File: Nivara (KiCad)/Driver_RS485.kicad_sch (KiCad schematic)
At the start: 3 parts

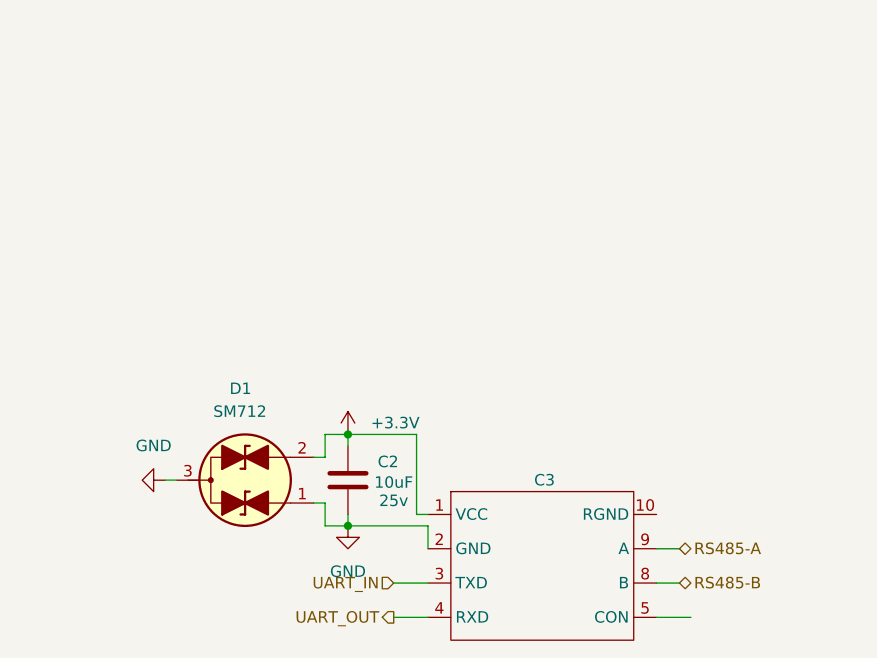
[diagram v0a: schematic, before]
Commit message: Add files via upload
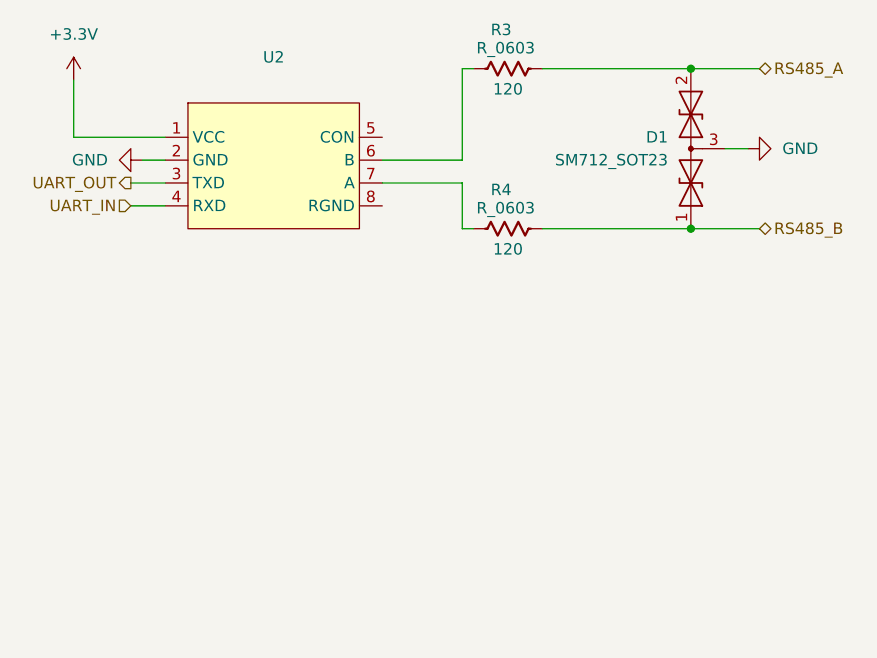
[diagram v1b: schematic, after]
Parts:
- removed C2: C_1206, PCM_Capacitor_SMD_AKL:C_1206_3216Metric, symbol PCM_Capacitor_US_AKL:C_1206
- removed C3: ~, RS485-MODULE:C2992406, symbol PCM_SL_Connectors:C2992406
- removed D1: SM712, PCM_Package_TO_SOT_SMD_AKL:SOT-23, symbol PCM_Diode_TVS_AKL:SM712
- added D1: SM712_SOT23, Package_TO_SOT_SMD:SOT-23_Handsoldering, symbol Diode:SM712_SOT23
- added R3, R4: R_0603, Resistor_SMD:R_0603_1608Metric, symbol PCM_Resistor_US_AKL:R_0603
- added U2: ~, External:RSM3485ECHT, symbol Proyecto_componente:RSM3485ECHT
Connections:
- net +3.3V: now also U2.1 (VCC)
- net GND: now also D1.3 (common), U2.2 (GND)
- net UART_IN: now also U2.4 (RXD)
- net UART_OUT: now also U2.3 (TXD)
- new net: R4.1, U2.7 (A)
- new net: R3.1, U2.6 (B)
- new net RS485_A: D1.2 (A2), R3.2
- new net RS485_B: D1.1 (A1), R4.2
